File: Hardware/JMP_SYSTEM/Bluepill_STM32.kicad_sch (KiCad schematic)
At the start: 2 parts, among them J1 BLUEPILL

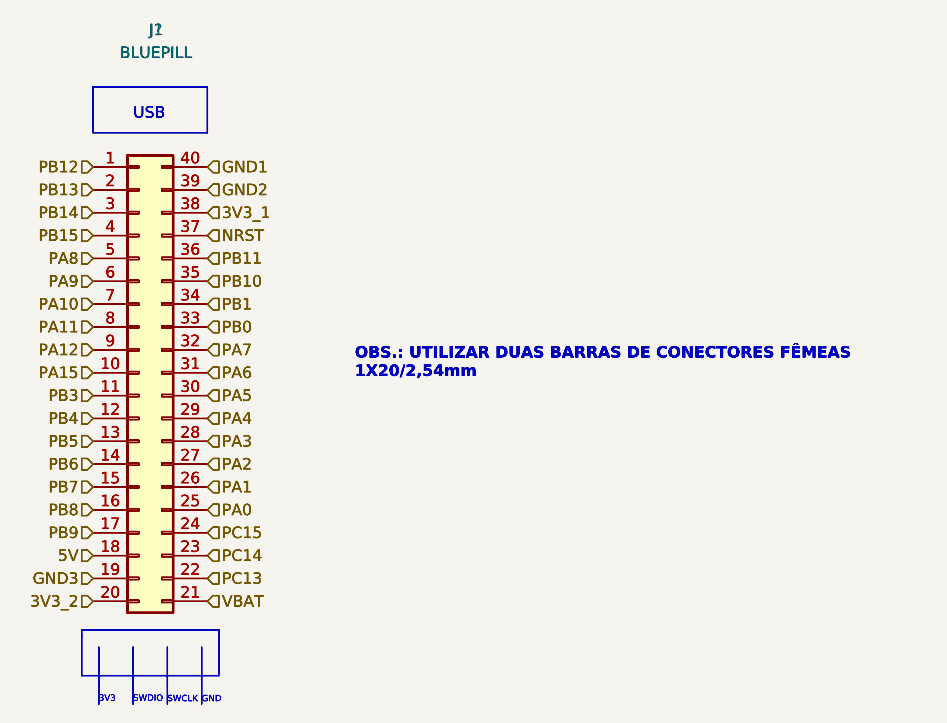
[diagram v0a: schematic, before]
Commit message: Schematics and PCB layout
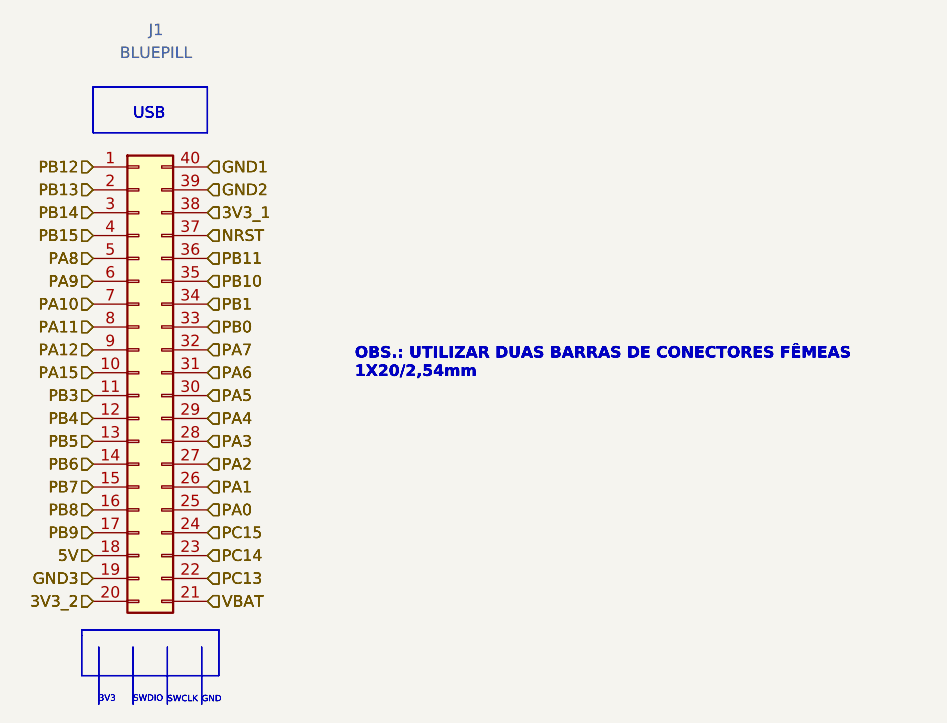
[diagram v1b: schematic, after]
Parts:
- removed J?: BLUEPILL, Package_DIP:DIP-40_W15.24mm_Socket_LongPads, symbol Connector_Generic:Conn_02x20_Counter_Clockwise
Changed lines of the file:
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@@
-    (pin "9")
-  )
-  (symbol (lib_id "Connector_Generic:Conn_02x20_Counter_Clockwise") (at 160.02 62.865 0) (unit 1)
-    (in_bom yes) (on_board yes)
-    (property "Reference" "J?" (id 0) (at 161.925 24.765 0))
-    (property "Value" "BLUEPILL" (id 1) (at 161.925 27.305 0))
-    (property "Footprint" "Package_DIP:DIP-40_W15.24mm_Socket_LongPads" (id 2) (at 161.925 29.845 0)
-      (effects (font (size 1.27 1.27)) hide)
-    )
-    (property "Datasheet" "~" (id 3) (at 160.02 62.865 0)
-      (effects (font (size 1.27 1.27)) hide)
-    )
-    (pin "1")
-    (pin "10")
-    (pin "11")
-    (pin "12")
-    (pin "13")
-    (pin "14")
-    (pin "15")
-    (pin "16")
-    (pin "17")
-    (pin "18")
-    (pin "19")
-    (pin "2")
-    (pin "20")
-    (pin "21")
-    (pin "22")
-    (pin "23")
-    (pin "24")
-    (pin "25")
-    (pin "26")
-    (pin "27")
-    (pin "28")
-    (pin "29")
-    (pin "3")
-    (pin "30")
-    (pin "31")
-    (pin "32")
-    (pin "33")
-    (pin "34")
-    (pin "35")
-    (pin "36")
-    (pin "37")
-    (pin "38")
-    (pin "39")
-    (pin "4")
-    (pin "40")
-    (pin "5")
-    (pin "6")
-    (pin "7")
-    (pin "8")
     (pin "9")
   )
